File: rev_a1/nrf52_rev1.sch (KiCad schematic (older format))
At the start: 31 parts, among them P1 CONN_01X18, P2 CONN_01X18, P3 USB_OTG, U1 nRF52832, U2 CP2102, U3 LT1129CST-3.3, Y1 32K, Y2 32M

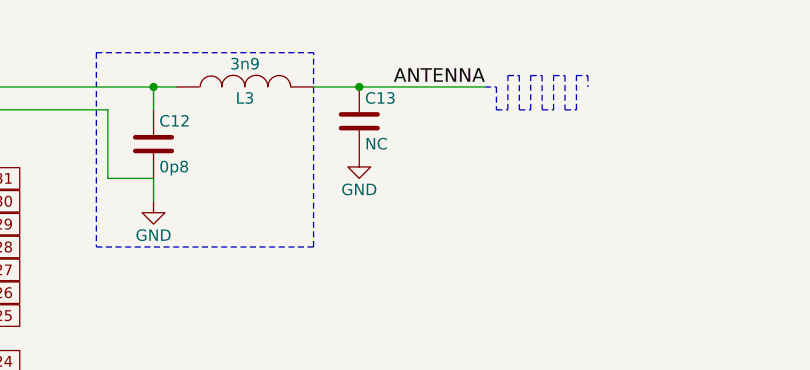
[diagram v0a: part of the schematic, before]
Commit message: wip
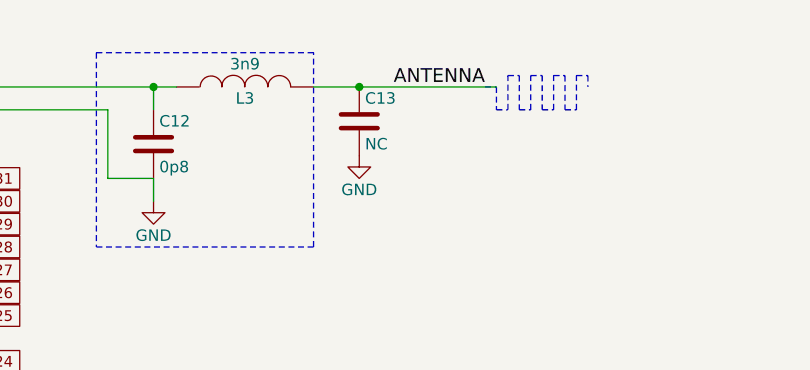
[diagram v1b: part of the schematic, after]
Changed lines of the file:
@@
 LIBS:tmp007
 LIBS:uvis25
+LIBS:tom_kicad
 LIBS:nrf52_rev1-cache
 EELAYER 25 0
@@
 	7000 650  6050 650
 Wire Wire Line
-	7000 800  7750 800
+	7000 800  7800 800
 Wire Notes Line
 	7750 800  7800 800

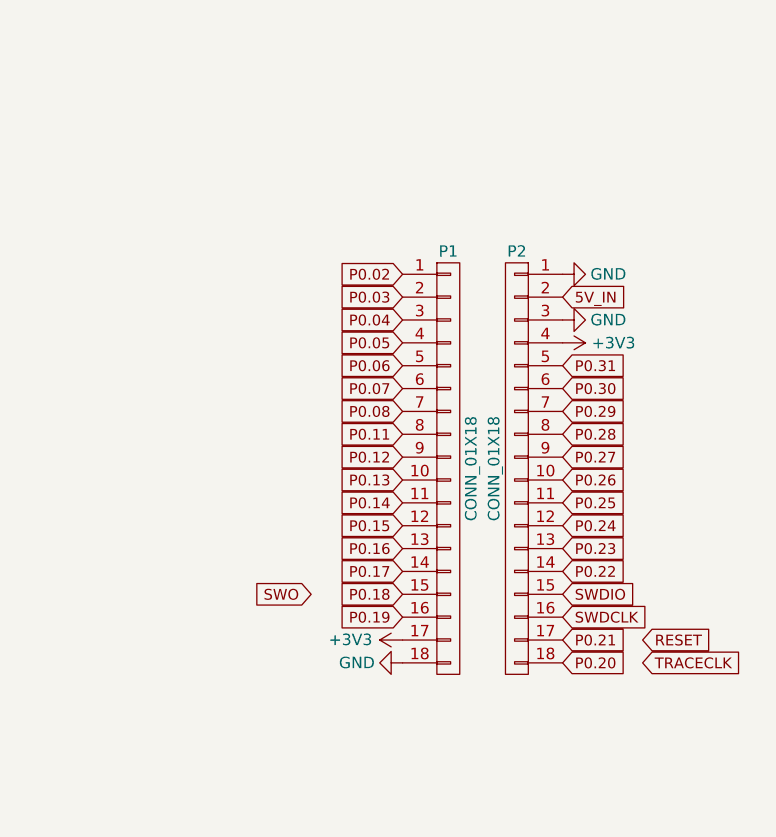
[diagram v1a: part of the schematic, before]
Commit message: wip
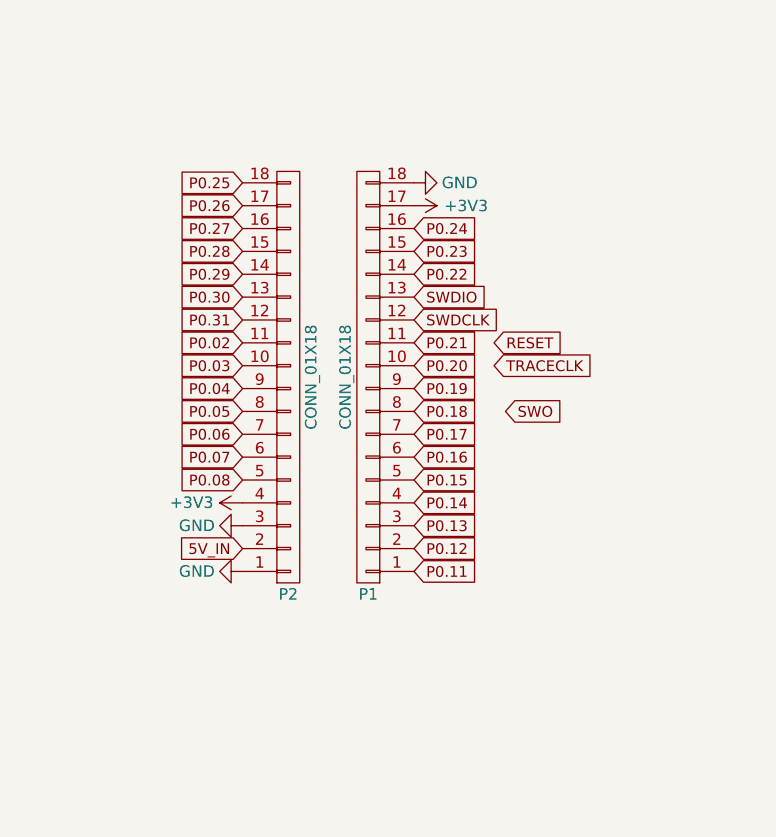
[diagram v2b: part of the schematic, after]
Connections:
- net P0.02: now also P2.11 (P11); no longer P1.1 (P1)
- net P0.03: now also P2.10 (P10); no longer P1.2 (P2)
- net P0.04: now also P2.9 (P9); no longer P1.3 (P3)
- net P0.05: now also P2.8 (P8); no longer P1.4 (P4)
- net P0.06: now also P2.7 (P7); no longer P1.5 (P5)
- net P0.07: now also P2.6 (P6); no longer P1.6 (P6)
- net P0.08: now also P2.5 (P5); no longer P1.7 (P7)
- net P0.11: now also P1.1 (P1); no longer P1.8 (P8)
- net P0.12: now also P1.2 (P2); no longer P1.9 (P9)
- net P0.13: now also P1.3 (P3); no longer P1.10 (P10)
- net P0.14: now also P1.4 (P4); no longer P1.11 (P11)
- net P0.15: now also P1.5 (P5); no longer P1.12 (P12)
- net P0.16: now also P1.6 (P6); no longer P1.13 (P13)
- net P0.17: now also P1.7 (P7); no longer P1.14 (P14)
- net P0.18: now also P1.8 (P8); no longer P1.15 (P15)
- net P0.19: now also P1.9 (P9); no longer P1.16 (P16)
- net P0.20: now also P1.10 (P10); no longer P2.18 (P18)
- net P0.21: now also P1.11 (P11); no longer P2.17 (P17)
- net P0.22: now also P1.14 (P14); no longer P2.14 (P14)
- net P0.23: now also P1.15 (P15); no longer P2.13 (P13)
- net P0.24: now also P1.16 (P16); no longer P2.12 (P12)
- net P0.25: now also P2.18 (P18); no longer P2.11 (P11)
- net P0.26: now also P2.17 (P17); no longer P2.10 (P10)
- net P0.27: now also P2.16 (P16); no longer P2.9 (P9)
- net P0.28: now also P2.15 (P15); no longer P2.8 (P8)
- net P0.29: now also P2.14 (P14); no longer P2.7 (P7)
- net P0.30: now also P2.13 (P13); no longer P2.6 (P6)
- net P0.31: now also P2.12 (P12); no longer P2.5 (P5)
- net SWDCLK: now also P1.12 (P12); no longer P2.16 (P16)
- net SWDIO: now also P1.13 (P13); no longer P2.15 (P15)
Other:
- moved on the sheet: P1, P2
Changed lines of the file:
@@
 LIBS:tmp007
 LIBS:uvis25
-LIBS:tom_kicad
 LIBS:nrf52_rev1-cache
 EELAYER 25 0
@@
 L CONN_01X18 P2
 U 1 1 57597D87
-P 9650 5400
-F 0 "P2" H 9650 6350 50  0000 C CNN
-F 1 "CONN_01X18" V 9750 5400 50  0000 C CNN
-F 2 "Pin_Headers:Pin_Header_Straight_1x18" H 9650 5400 50  0001 C CNN
-F 3 "" H 9650 5400 50  0000 C CNN
-	1    9650 5400
-	-1   0    0    -1
+P 8650 5000
+F 0 "P2" H 8650 5950 50  0000 C CNN
+F 1 "CONN_01X18" V 8750 5000 50  0000 C CNN
+F 2 "Pin_Headers:Pin_Header_Straight_1x18" H 8650 5000 50  0001 C CNN
+F 3 "" H 8650 5000 50  0000 C CNN
+	1    8650 5000
+	1    0    0    1
 $EndComp
 $Comp
 L CONN_01X18 P1
 U 1 1 57597D15
-P 9350 5400
-F 0 "P1" H 9350 6350 50  0000 C CNN
-F 1 "CONN_01X18" V 9450 5400 50  0000 C CNN
-F 2 "Pin_Headers:Pin_Header_Straight_1x18" H 9350 5400 50  0001 C CNN
-F 3 "" H 9350 5400 50  0000 C CNN
-	1    9350 5400
-	1    0    0    -1
+P 9000 5000
+F 0 "P1" H 9000 5950 50  0000 C CNN
+F 1 "CONN_01X18" V 9100 5000 50  0000 C CNN
+F 2 "Pin_Headers:Pin_Header_Straight_1x18" H 9000 5000 50  0001 C CNN
+F 3 "" H 9000 5000 50  0000 C CNN
+	1    9000 5000
+	-1   0    0    1
 $EndComp
 $Comp
@@
 	1    0    0    -1
 $EndComp
-Text GLabel 9850 4650 2    47   Input ~ 0
+Text GLabel 8450 5750 0    47   Input ~ 0
 5V_IN
 $Comp
@@
 	-1   0    0    1
 $EndComp
-Text GLabel 9150 5850 0    47   Input ~ 0
+Text GLabel 9200 5250 2    47   Input ~ 0
 P0.17
-Text GLabel 9150 5750 0    47   Input ~ 0
+Text GLabel 9200 5350 2    47   Input ~ 0
 P0.16
-Text GLabel 9150 5650 0    47   Input ~ 0
+Text GLabel 9200 5450 2    47   Input ~ 0
 P0.15
-Text GLabel 9150 5550 0    47   Input ~ 0
+Text GLabel 9200 5550 2    47   Input ~ 0
 P0.14
-Text GLabel 9150 5450 0    47   Input ~ 0
+Text GLabel 9200 5650 2    47   Input ~ 0
 P0.13
-Text GLabel 9150 5350 0    47   Input ~ 0
+Text GLabel 9200 5750 2    47   Input ~ 0
 P0.12
-Text GLabel 9150 5250 0    47   Input ~ 0
+Text GLabel 9200 5850 2    47   Input ~ 0
 P0.11
-Text GLabel 9150 4550 0    47   Input ~ 0
+Text GLabel 8450 4850 0    47   Input ~ 0
 P0.02
-Text GLabel 9150 4650 0    47   Input ~ 0
+Text GLabel 8450 4950 0    47   Input ~ 0
 P0.03
-Text GLabel 9150 4750 0    47   Input ~ 0
+Text GLabel 8450 5050 0    47   Input ~ 0
 P0.04
-Text GLabel 9150 4850 0    47   Input ~ 0
+Text GLabel 8450 5150 0    47   Input ~ 0
 P0.05
-Text GLabel 9150 4950 0    47   Input ~ 0
+Text GLabel 8450 5250 0    47   Input ~ 0
 P0.06
-Text GLabel 9150 6050 0    47   Input ~ 0
+Text GLabel 9200 5050 2    47   Input ~ 0
 P0.19
-Text GLabel 9850 6250 2    47   Input ~ 0
+Text GLabel 9200 4950 2    47   Input ~ 0
 P0.20
-Text GLabel 9850 6150 2    47   Input ~ 0
+Text GLabel 9200 4850 2    47   Input ~ 0
 P0.21
-Text GLabel 9850 5850 2    47   Input ~ 0
+Text GLabel 9200 4550 2    47   Input ~ 0
 P0.22
-Text GLabel 9850 5750 2    47   Input ~ 0
+Text GLabel 9200 4450 2    47   Input ~ 0
 P0.23
-Text GLabel 9850 5650 2    47   Input ~ 0
+Text GLabel 9200 4350 2    47   Input ~ 0
 P0.24
-Text GLabel 9850 5550 2    47   Input ~ 0
+Text GLabel 8450 4150 0    47   Input ~ 0
 P0.25
-Text GLabel 9850 5450 2    47   Input ~ 0
+Text GLabel 8450 4250 0    47   Input ~ 0
 P0.26
-Text GLabel 9850 5350 2    47   Input ~ 0
+Text GLabel 8450 4350 0    47   Input ~ 0
 P0.27
-Text GLabel 9850 5250 2    47   Input ~ 0
+Text GLabel 8450 4450 0    47   Input ~ 0
 P0.28
-Text GLabel 9850 5150 2    47   Input ~ 0
+Text GLabel 8450 4550 0    47   Input ~ 0
 P0.29
-Text GLabel 9850 5050 2    47   Input ~ 0
+Text GLabel 8450 4650 0    47   Input ~ 0
 P0.30
-Text GLabel 9150 5950 0    47   Input ~ 0
+Text GLabel 9200 5150 2    47   Input ~ 0
 P0.18
-Text GLabel 9850 4950 2    47   Input ~ 0
+Text GLabel 8450 4750 0    47   Input ~ 0
 P0.31
 Text GLabel 3250 2300 0    47   Input ~ 0
@@
 Text GLabel 3250 1900 0    47   Input ~ 0
 XC2
-Text GLabel 9850 5950 2    47   Input ~ 0
+Text GLabel 9200 4650 2    47   Input ~ 0
 SWDIO
-Text GLabel 9850 6050 2    47   Input ~ 0
+Text GLabel 9200 4750 2    47   Input ~ 0
 SWDCLK
 Text GLabel 6250 2500 2    47   Input ~ 0
@@
 Text Notes 6300 2200 0    60   ~ 0
 Debug interface
-Text GLabel 10200 6250 2    47   Input ~ 0
+Text GLabel 9550 4950 2    47   Input ~ 0
 TRACECLK
-Text GLabel 10200 6150 2    47   Input ~ 0
+Text GLabel 9550 4850 2    47   Input ~ 0
 RESET
-Text GLabel 8750 5950 0    47   Input ~ 0
+Text GLabel 9600 5150 2    47   Input ~ 0
 SWO
 $Comp
 L GND #PWR030
 U 1 1 575DC1F5
-P 9150 6250
-F 0 "#PWR030" H 9150 6000 50  0001 C CNN
-F 1 "GND" V 9150 6050 50  0000 C CNN
-F 2 "" H 9150 6250 50  0000 C CNN
-F 3 "" H 9150 6250 50  0000 C CNN
-	1    9150 6250
-	0    1    1    0
+P 9200 4150
+F 0 "#PWR030" H 9200 3900 50  0001 C CNN
+F 1 "GND" V 9200 3950 50  0000 C CNN
+F 2 "" H 9200 4150 50  0000 C CNN
+F 3 "" H 9200 4150 50  0000 C CNN
+	1    9200 4150
+	0    -1   -1   0
 $EndComp
 $Comp
 L +3V3 #PWR031
 U 1 1 575DC6AD
-P 9150 6150
-F 0 "#PWR031" H 9150 6000 50  0001 C CNN
-F 1 "+3V3" V 9151 6378 50  0000 C CNN
-F 2 "" H 9150 6150 50  0000 C CNN
-F 3 "" H 9150 6150 50  0000 C CNN
-	1    9150 6150
-	0    -1   -1   0
+P 9200 4250
+F 0 "#PWR031" H 9200 4100 50  0001 C CNN
+F 1 "+3V3" V 9201 4478 50  0000 C CNN
+F 2 "" H 9200 4250 50  0000 C CNN
+F 3 "" H 9200 4250 50  0000 C CNN
+	1    9200 4250
+	0    1    1    0
 $EndComp
 $Comp
 L GND #PWR032
 U 1 1 575DC996
-P 9850 4550
-F 0 "#PWR032" H 9850 4300 50  0001 C CNN
-F 1 "GND" V 9850 4350 50  0000 C CNN
-F 2 "" H 9850 4550 50  0000 C CNN
-F 3 "" H 9850 4550 50  0000 C CNN
-	1    9850 4550
-	0    -1   1    0
+P 8450 5850
+F 0 "#PWR032" H 8450 5600 50  0001 C CNN
+F 1 "GND" V 8450 5650 50  0000 C CNN
+F 2 "" H 8450 5850 50  0000 C CNN
+F 3 "" H 8450 5850 50  0000 C CNN
+	1    8450 5850
+	0    1    -1   0
 $EndComp
 $Comp
 L +3V3 #PWR033
 U 1 1 575DCAE2
-P 9850 4850
-F 0 "#PWR033" H 9850 4700 50  0001 C CNN
-F 1 "+3V3" V 9849 5073 50  0000 C CNN
-F 2 "" H 9850 4850 50  0000 C CNN
-F 3 "" H 9850 4850 50  0000 C CNN
-	1    9850 4850
-	0    1    -1   0
+P 8450 5550
+F 0 "#PWR033" H 8450 5400 50  0001 C CNN
+F 1 "+3V3" V 8449 5773 50  0000 C CNN
+F 2 "" H 8450 5550 50  0000 C CNN
+F 3 "" H 8450 5550 50  0000 C CNN
+	1    8450 5550
+	0    -1   1    0
 $EndComp
 $Comp
 L GND #PWR034
 U 1 1 575DCBF4
-P 9850 4750
-F 0 "#PWR034" H 9850 4500 50  0001 C CNN
-F 1 "GND" V 9850 4550 50  0000 C CNN
-F 2 "" H 9850 4750 50  0000 C CNN
-F 3 "" H 9850 4750 50  0000 C CNN
-	1    9850 4750
-	0    -1   1    0
-$EndComp
-Text GLabel 9150 5150 0    47   Input ~ 0
+P 8450 5650
+F 0 "#PWR034" H 8450 5400 50  0001 C CNN
+F 1 "GND" V 8450 5450 50  0000 C CNN
+F 2 "" H 8450 5650 50  0000 C CNN
+F 3 "" H 8450 5650 50  0000 C CNN
+	1    8450 5650
+	0    1    -1   0
+$EndComp
+Text GLabel 8450 5450 0    47   Input ~ 0
 P0.08
-Text GLabel 9150 5050 0    47   Input ~ 0
+Text GLabel 8450 5350 0    47   Input ~ 0
 P0.07
 $Comp
